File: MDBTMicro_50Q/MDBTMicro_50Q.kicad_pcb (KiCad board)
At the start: 2 copper layers, 33.3 x 18 mm, 37 parts, among them J1 ProMicro Pinout, J2 USB_C_Receptacle_USB2.0, Q1 AO3407, Q2 AO3407, U1 XC6220B331MR-G, U2 MDBT50Q-x1MV2, U3 TP4057, X1 32.768kHz

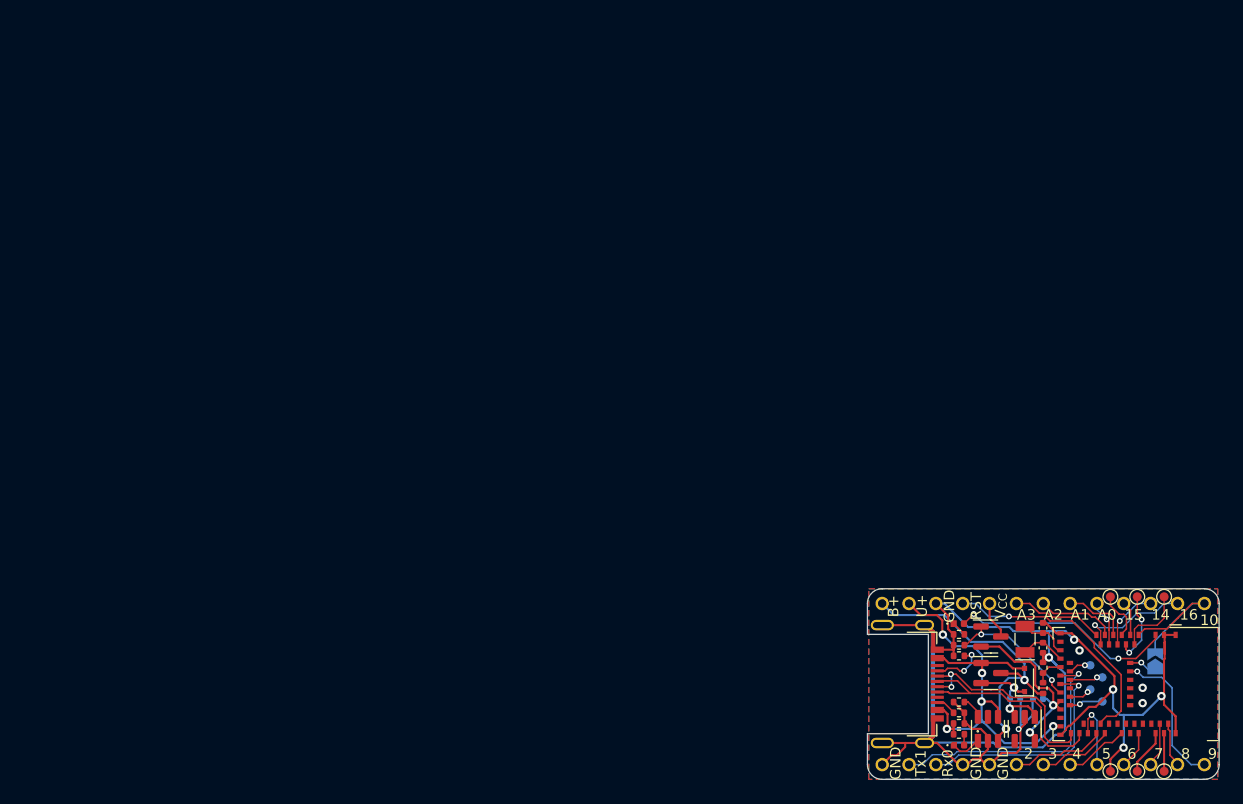
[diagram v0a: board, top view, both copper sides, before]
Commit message: Update 1.2
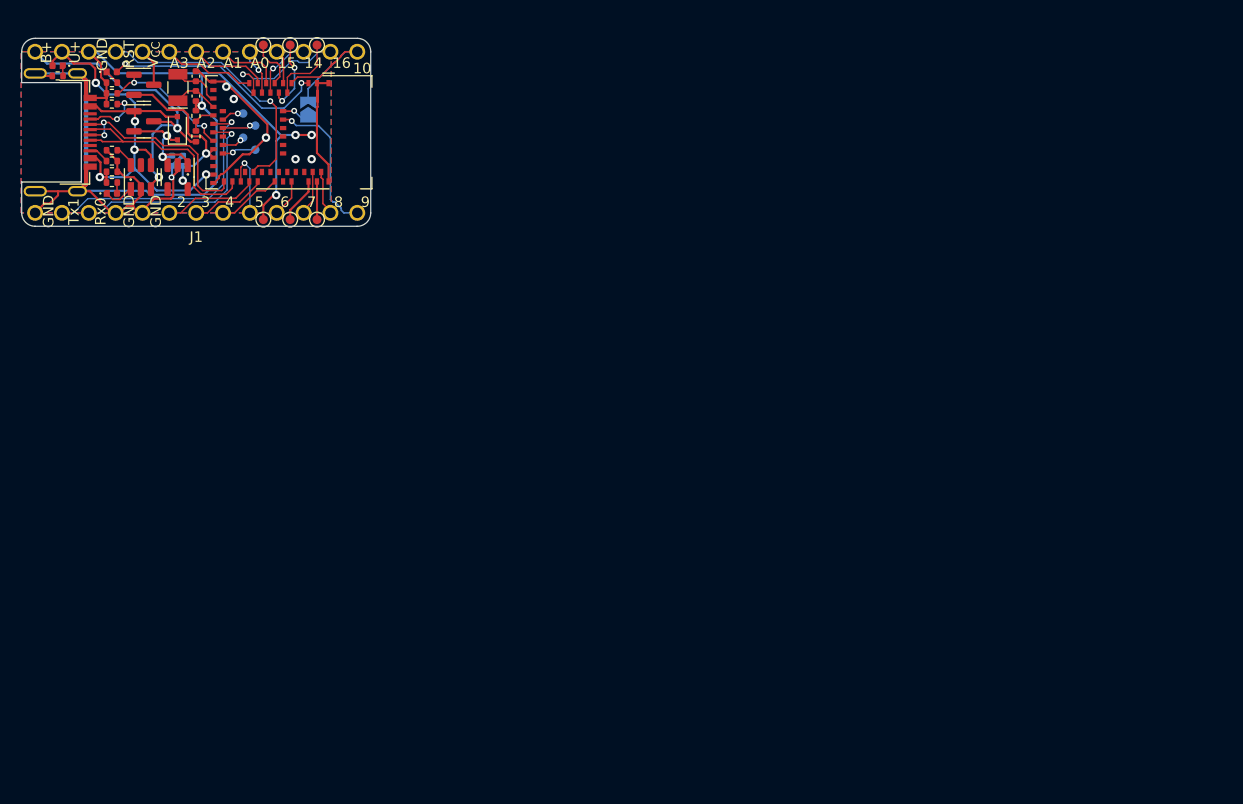
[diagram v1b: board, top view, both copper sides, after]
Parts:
- added LD3: Green, LED_SMD:LED_0402_1005Metric, F.Cu at (54.1, 43.1)
- added R5: 1k, Resistor_SMD:R_0402_1005Metric, F.Cu at (54.1, 44.1)
- J1: footprint MDBTMicro_library:ProMicro -> MDBTMicro_library:ProMicro board pinout
- J2: value USB_C_Receptacle_USB2.0 -> USB_C
- LD1: value Charging -> Red
- LD2: value User -> Blue
- moved ? 95.6 mm to (51.9, 57.0)
- moved ? 95.6 mm to (51.9, 41.8)
- moved C4 95.6 mm to (67.2, 46.0)
- moved R9 95.6 mm to (59.2, 46.7)
- moved TP2 95.6 mm to (76.1, 41.1)
- moved TP9 95.6 mm to (76.1, 57.7)
- moved U3 95.6 mm to (62.0, 53.6)
- moved X1 95.6 mm to (65.5, 45.2)
- moved C3 95.6 mm to (67.2, 44.1)
- moved D1 95.6 mm to (65.4, 49.0)
- moved J2 95.6 mm to (52.9, 49.4)
- moved JP1 95.6 mm to (77.8, 47.3)
- moved LD1 95.6 mm to (59.2, 55.2)
- moved LD2 95.6 mm to (59.2, 43.7)
- moved Q1 95.6 mm to (62.2, 48.4)
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- renumbered R9 to R10, R5 to R6, R6 to R7, R7 to R8, R8 to R9
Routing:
- net GND: track 148.9 -> 154.3 mm, vias 9 -> 10
- net VBUS: track 45.8 -> 47.5 mm
- net /P0.28: track 10.9 -> 12.1 mm
- net RESET: track 24.0 -> 25.0 mm
- net Net-(LD3-Pad1): track 0.00 -> 1.03 mm
- net Net-(C1-Pad1): track 10.4 -> 11.3 mm
- net nRF_VDD: track 18.2 -> 17.6 mm
- net /P0.06: track 24.9 -> 24.4 mm
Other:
- board size 33.3 x 18 mm -> 33 x 17.8 mm
- board text added: "MDBTMicro 50Q v1.2"
- board text removed: "MDBTMicro 50Q v1.1"

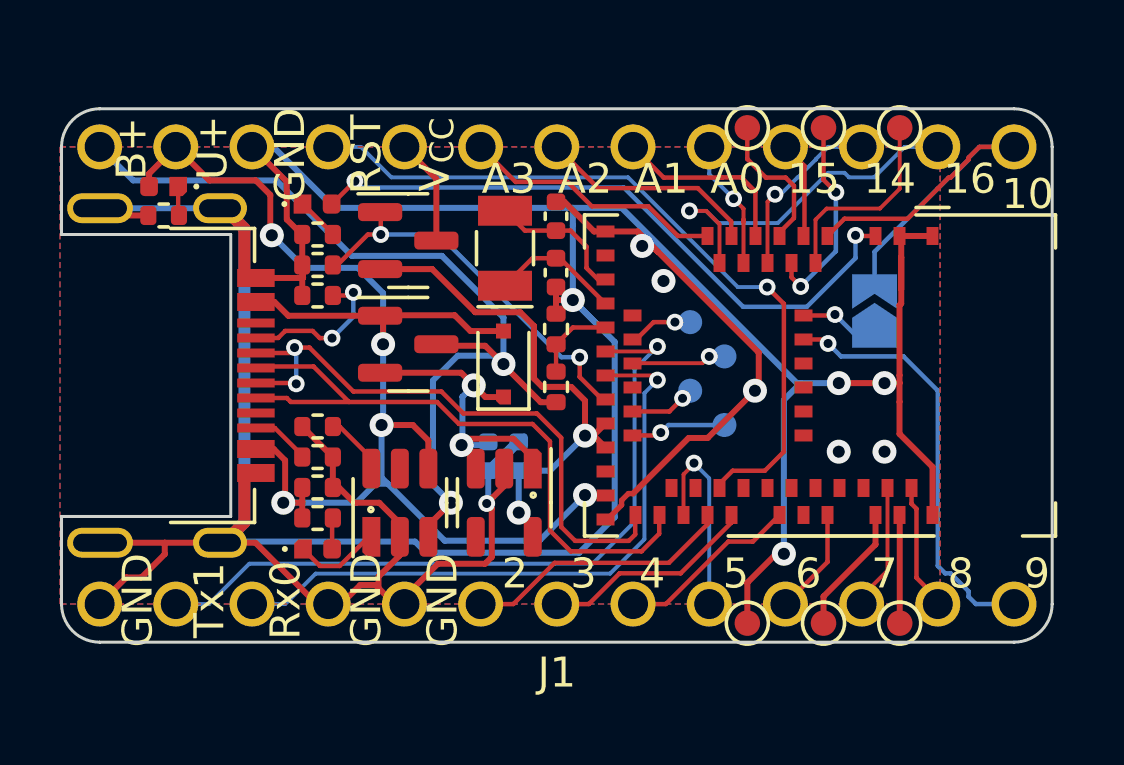
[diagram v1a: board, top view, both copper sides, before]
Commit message: Update 1.3
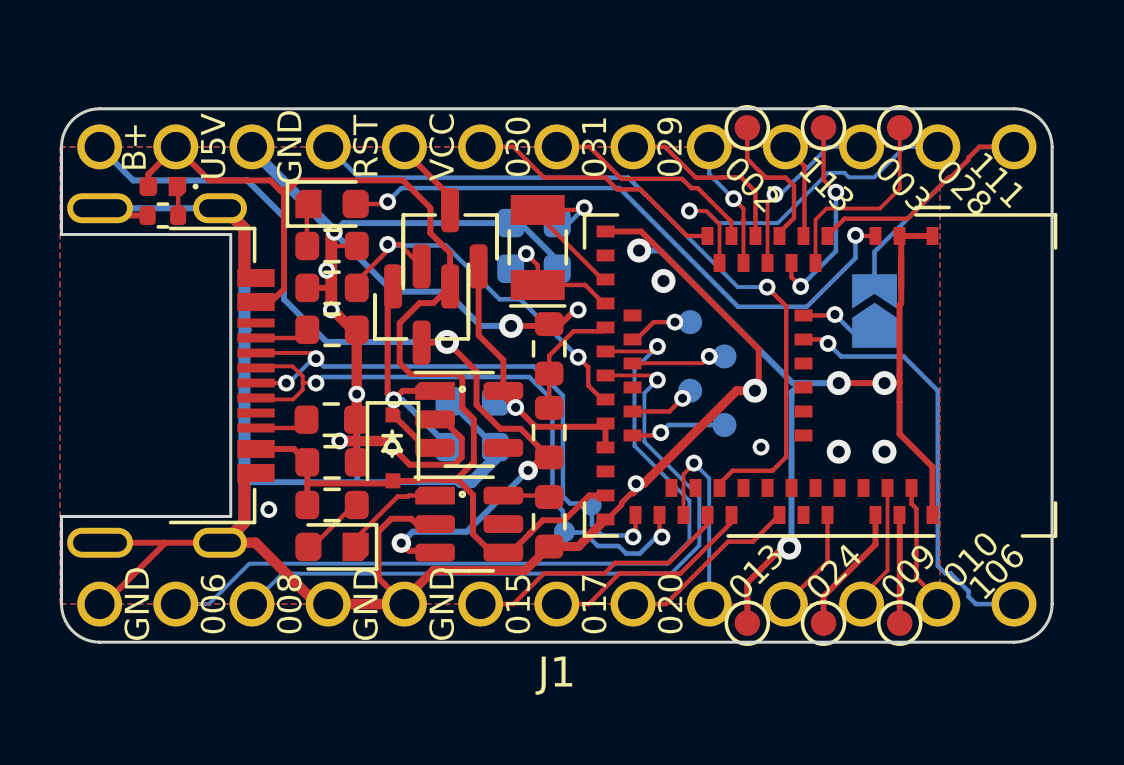
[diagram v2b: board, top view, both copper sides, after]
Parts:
- added REF**: TestPoint_Pad_D1.0mm, TestPoint:TestPoint_Pad_D1.0mm, B.Cu at (68.3, 53.7)
- added REF**: TestPoint_Pad_D1.0mm, TestPoint:TestPoint_Pad_D1.0mm, B.Cu at (67.4, 54.6)
- C1, C2: footprint Capacitor_SMD:C_0402_1005Metric -> Capacitor_SMD:C_0603_1608Metric
- C3, C4: footprint Capacitor_SMD:C_0402_1005Metric -> Capacitor_SMD:C_0603_1608Metric; moved to B.Cu
- J2: value USB_C -> USB_C_Receptacle_USB2.0
- LD1, LD2: footprint LED_SMD:LED_0402_1005Metric -> LED_SMD:LED_0603_1608Metric
- R1, R10, R2, R3, R4, R6, R7, R8, R9: footprint Resistor_SMD:R_0402_1005Metric -> Resistor_SMD:R_0603_1608Metric
- moved R3 8.35 mm to (66.9, 54.3), turned to 90 degrees
- moved D1 4.62 mm to (61.7, 51.8), turned to -90 degrees
- moved U1 3.01 mm to (64.3, 50.9), turned to 0 degrees
- moved U3 2.42 mm to (64.3, 54.4), turned to 0 degrees
- moved C2 2.40 mm to (64.4, 50.3), turned to 180 degrees
- moved R6 1.54 mm to (66.9, 51.3)
- moved Q2 1.40 mm to (63.6, 44.8), turned to 90 degrees
- moved R10 1.33 mm to (59.7, 50.9)
- moved R9 1.24 mm to (59.7, 47.9), turned to 0 degrees
- moved X1 1.09 mm to (66.5, 45.1)
- moved Q1 1.09 mm to (62.7, 47.4), turned to -90 degrees
- moved R1 0.97 mm to (59.7, 52.3)
- moved R8 0.90 mm to (59.7, 46.5)
- moved C3 0.77 mm to (66.4, 44.3), turned to 0 degrees
- moved C4 0.75 mm to (66.4, 45.8), turned to 180 degrees
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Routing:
- net nRF_VDD: track 17.6 -> 10.7 mm, vias 2 -> 1
- net GND: track 154.3 -> 150.5 mm, vias 10 -> 19
- net Net-(J2-PadA5): track 5.48 -> 2.03 mm, vias 2 -> 0
- net /P0.06: track 24.4 -> 27.4 mm
- net /P0.08: track 21.3 -> 24.0 mm
- net VBUS: track 47.5 -> 45.3 mm, vias 5 -> 0
- net VBAT: track 31.1 -> 29.8 mm, vias 2 -> 3
- net Net-(C3-Pad2): track 4.71 -> 5.99 mm, vias 0 -> 1
- net BATTERY_PIN: track 2.82 -> 4.01 mm
- net Net-(LD1-Pad2): track 1.04 -> 2.19 mm
- net Net-(C1-Pad1): track 11.3 -> 10.3 mm, vias 2 -> 1
- net LED_PIN: track 21.6 -> 20.6 mm
- net EXT_VCC: track 3.54 -> 2.74 mm
- net Net-(LD1-Pad1): track 2.92 -> 3.52 mm
- net Net-(R3-Pad2): track 2.06 -> 1.55 mm
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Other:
- board text added: "002"
- board text added: "003"
- board text added: "005"
- board text added: "007"
- board text added: "008"
- board text added: "009"
- board text added: "010"
- board text added: "011"
- board text added: "012"
- board text added: "013"
- board text added: "015"
- board text added: "017"
- board text added: "020"
- board text added: "024"
- board text added: "028"
- board text added: "029"
- board text added: "030"
- board text added: "031"
- board text added: "106"
- board text added: "111"
- board text added: "112"
- board text added: "113"
- board text added: "114"
- board text added: "115"
- board text added: "B +"
- board text added: "G"
- board text added: "MDBTMicro 50Q"
- board text added: "SWC"
- board text added: "SWD"
- board text added: "U5V"
- board text added: "VCC"
- board text added: "v1.3"
- board text removed: "0.02"
- board text removed: "0.03"
- board text removed: "0.08"
- board text removed: "0.09"
- board text removed: "0.10"
- board text removed: "0.13"
- board text removed: "0.15"
- board text removed: "0.17"
- board text removed: "0.18"
- board text removed: "0.20"
- board text removed: "0.24"
- board text removed: "0.28"
- board text removed: "0.29"
- board text removed: "0.30"
- board text removed: "0.31"
- board text removed: "1.06"
- board text removed: "1.11"
- board text removed: "1.13"
- board text removed: "MDBTMicro 50Q v1.2"
- board text removed: "U+"
- board text removed: "V_{CC}"
